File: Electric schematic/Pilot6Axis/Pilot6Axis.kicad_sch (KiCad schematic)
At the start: 63 parts, among them IC1 ESP32-WROOM-32U, IC2 LM27313XMFX_NOPB, J1 BTN1, J10 Power switch, J11 TP4056, J12 OLED, J13 USB_C_Receptacle_USB2.0_16P, J14 BTN9, J15 BTN11, J16 BTN10, J2 BTN2, J3 BTN3, J4 BTN4, J5 BTN5, J6 BTN6, J7 BTN7, J8 BTN8, J9 BAT, Q1 Q_NPN_EBC, Q2 Q_NPN_EBC, SW1 SW_Push, SW2 SW_Push, U1 JOYSTICK1, U2 JOYSTICK2, U3 AMS1117-3.3, U4 USBLC6-2SC6, U5 CP2102N-Axx-xQFN28

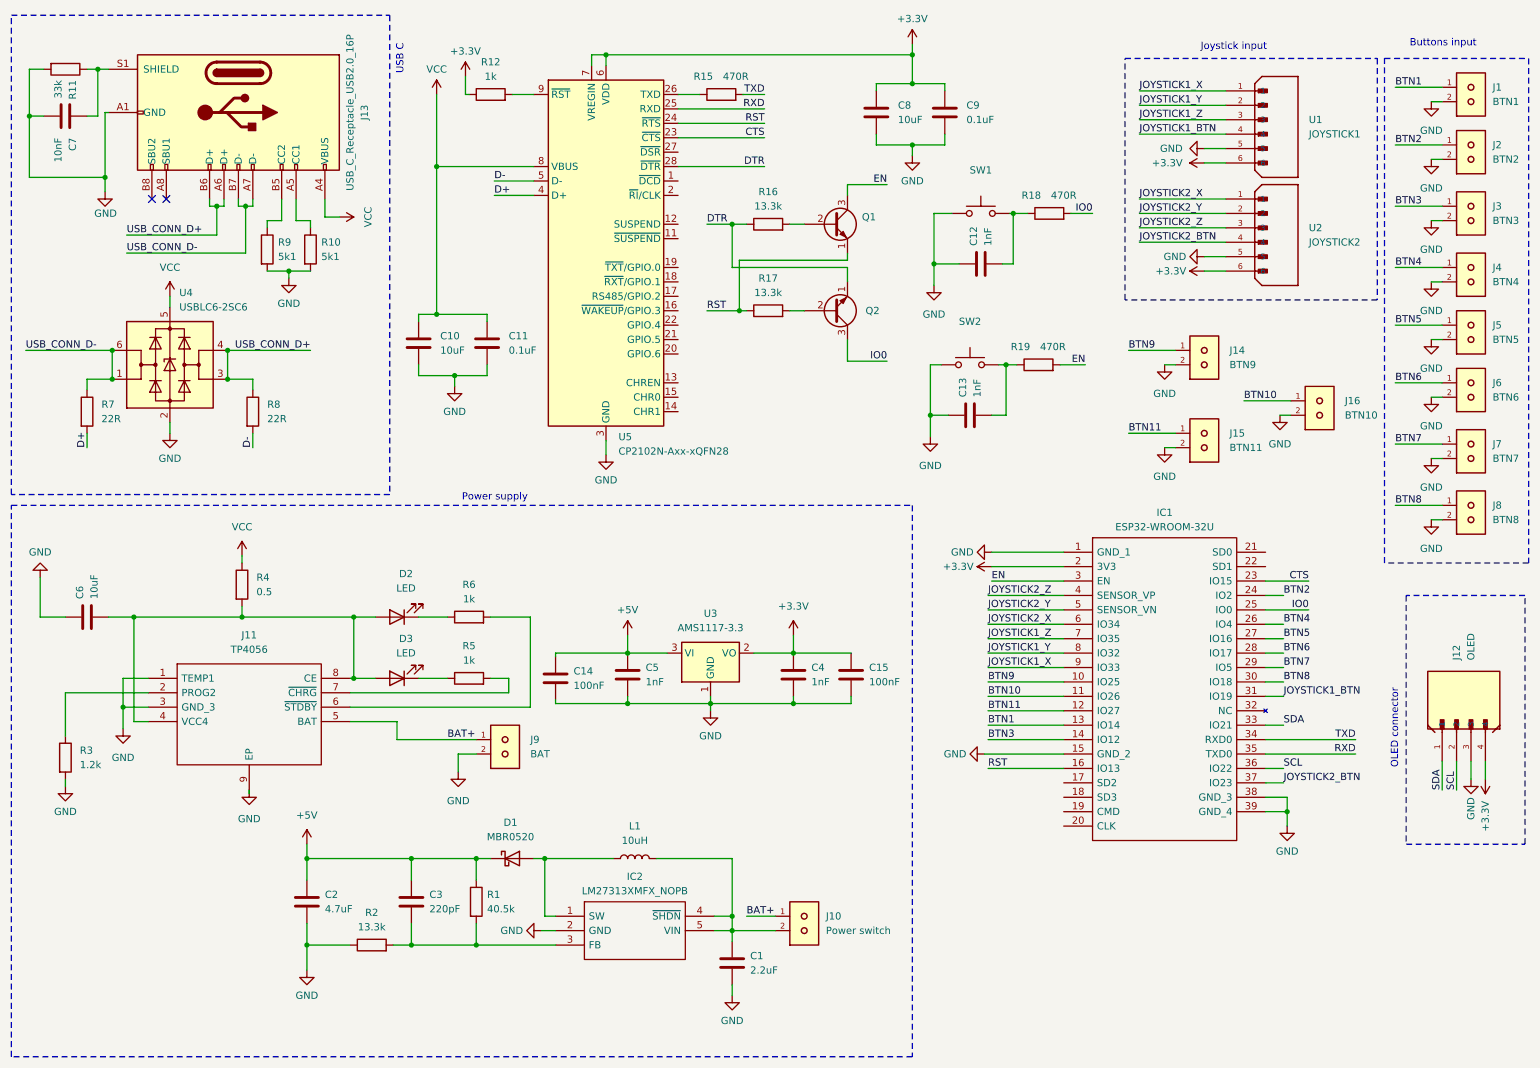
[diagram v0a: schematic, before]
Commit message: Update pilot PCB versin 1.0
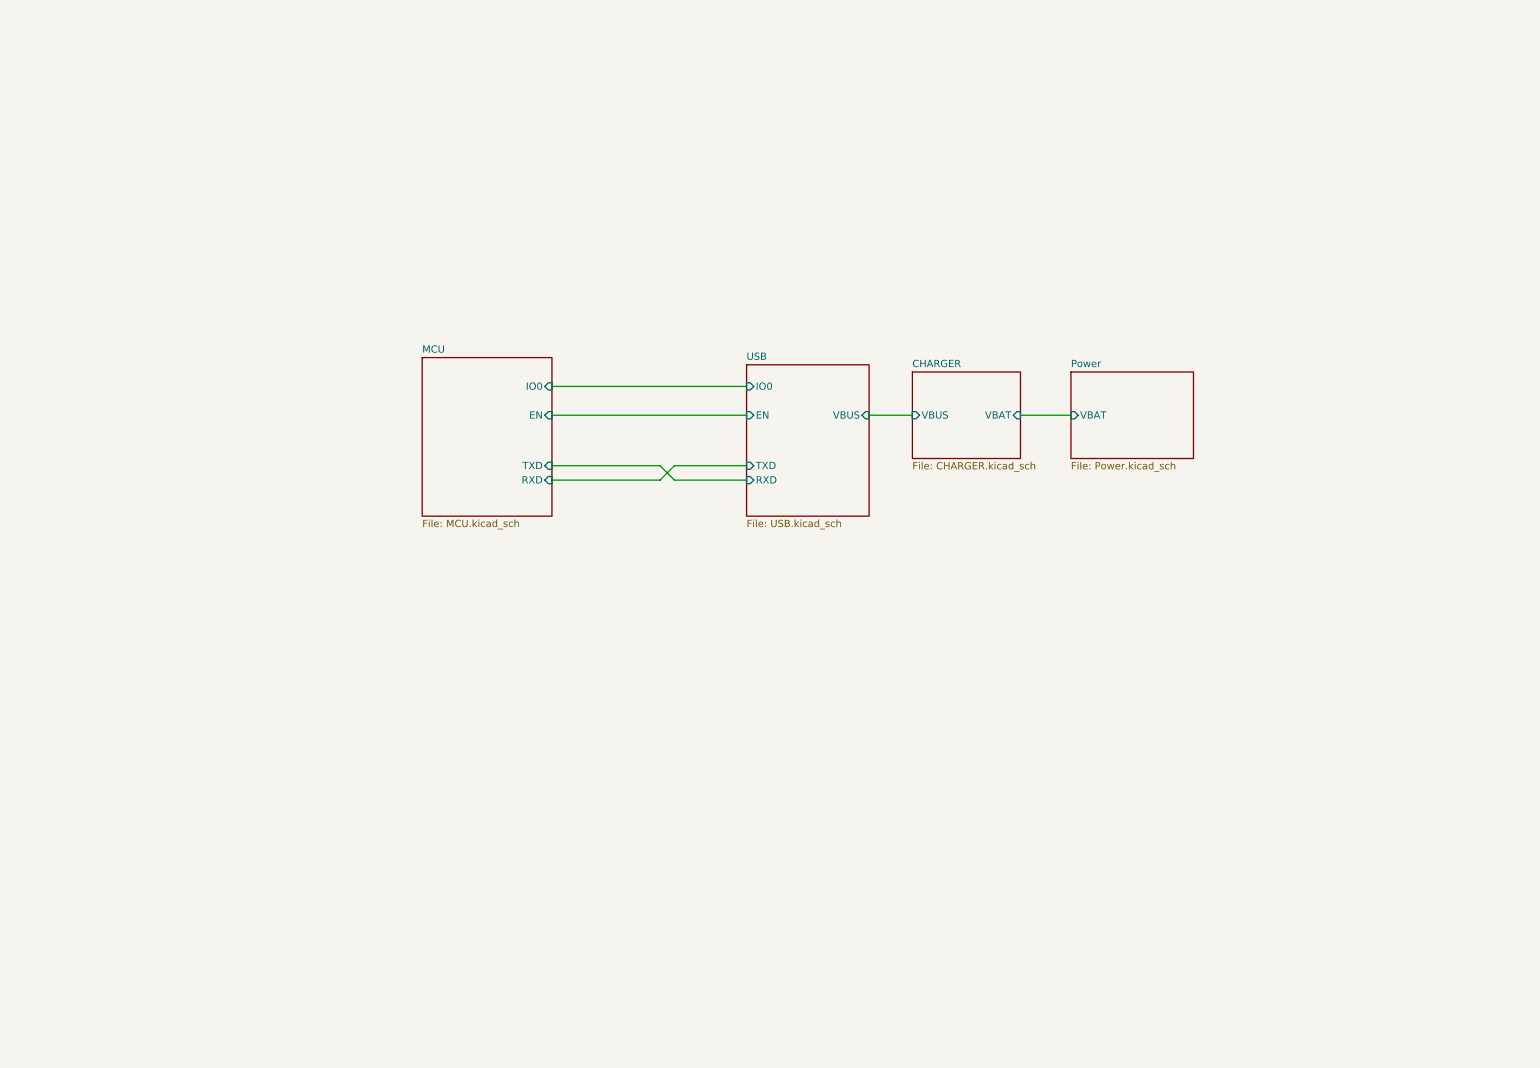
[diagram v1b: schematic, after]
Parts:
- removed C1: 2.2uF, Capacitor_SMD:C_0603_1608Metric, symbol Device:C
- removed C10, C8: 10uF, Resistor_SMD:R_0603_1608Metric, symbol Device:C
- removed C11, C9: 0.1uF, Resistor_SMD:R_0603_1608Metric, symbol Device:C
- removed C12, C13, C4, C5: 1nF, Capacitor_SMD:C_0603_1608Metric, symbol Device:C
- removed C14, C15: 100nF, Capacitor_SMD:C_0603_1608Metric, symbol Device:C
- removed C2: 4.7uF, Capacitor_SMD:C_0603_1608Metric, symbol Device:C
- removed C3: 220pF, Capacitor_SMD:C_0603_1608Metric, symbol Device:C
- removed C6: 10uF, Capacitor_SMD:C_0603_1608Metric, symbol Device:C
- removed C7: 10nF, Resistor_SMD:R_0603_1608Metric, symbol Device:C
- removed D1: MBR0520, Diode_SMD:D_0603_1608Metric, symbol Device:D_Schottky
- removed D2, D3: LED, LED_SMD:LED_0603_1608Metric, symbol Device:LED
- removed IC1: ESP32-WROOM-32U, ESP32-WROOM-32U:ESP32WROOM32D, symbol ESP32-WROOM-32U:ESP32-WROOM-32U
- removed IC2: LM27313XMFX_NOPB, KLM27313XMF_NOPB:SOT95P280X145-5N, symbol LM27313XMFX_NOPB:LM27313XMFX_NOPB
- removed J1: BTN1, molex-2pin:HDRV2W64P254_1X2_580X508X1170P, symbol molex-2pin:22-27-2021
- removed J10: Power switch, molex-2pin:HDRV2W64P254_1X2_580X508X1170P, symbol molex-2pin:22-27-2021
- removed J11: TP4056, TP4056:SOIC127P600X175-9N, symbol TP4056:TP4056
- removed J12: OLED, Connector_PinSocket_2.54mm:PinSocket_2x02_P2.54mm_Vertical, symbol molex-4pin:22232041
- removed J13: USB_C_Receptacle_USB2.0_16P, Connector_USB:USB_C_Receptacle_HCTL_HC-TYPE-C-16P-01A, symbol Connector:USB_C_Receptacle_USB2.0_16P
- removed J14: BTN9, molex-2pin:HDRV2W64P254_1X2_580X508X1170P, symbol molex-2pin:22-27-2021
- removed J15: BTN11, molex-2pin:HDRV2W64P254_1X2_580X508X1170P, symbol molex-2pin:22-27-2021
- removed J16: BTN10, molex-2pin:HDRV2W64P254_1X2_580X508X1170P, symbol molex-2pin:22-27-2021
- removed J2: BTN2, molex-2pin:HDRV2W64P254_1X2_580X508X1170P, symbol molex-2pin:22-27-2021
- removed J3: BTN3, molex-2pin:HDRV2W64P254_1X2_580X508X1170P, symbol molex-2pin:22-27-2021
- removed J4: BTN4, molex-2pin:HDRV2W64P254_1X2_580X508X1170P, symbol molex-2pin:22-27-2021
- removed J5: BTN5, molex-2pin:HDRV2W64P254_1X2_580X508X1170P, symbol molex-2pin:22-27-2021
- removed J6: BTN6, molex-2pin:HDRV2W64P254_1X2_580X508X1170P, symbol molex-2pin:22-27-2021
- removed J7: BTN7, molex-2pin:HDRV2W64P254_1X2_580X508X1170P, symbol molex-2pin:22-27-2021
- removed J8: BTN8, molex-2pin:HDRV2W64P254_1X2_580X508X1170P, symbol molex-2pin:22-27-2021
- removed J9: BAT, molex-2pin:HDRV2W64P254_1X2_580X508X1170P, symbol molex-2pin:22-27-2021
- removed L1: 10uH, Inductor_SMD:L_APV_ANR4010, symbol Device:L
- removed Q1, Q2: Q_NPN_EBC, S8050:SOT95P240X115-3N, symbol Device:Q_NPN_EBC
- removed R1: 40.5k, Resistor_SMD:R_0603_1608Metric, symbol Device:R
- removed R10, R9: 5k1, Resistor_SMD:R_0603_1608Metric, symbol Device:R
- removed R11: 33k, Resistor_SMD:R_0603_1608Metric, symbol Device:R
- removed R12, R5, R6: 1k, Resistor_SMD:R_0603_1608Metric, symbol Device:R
- removed R15, R18, R19: 470R, Resistor_SMD:R_0603_1608Metric, symbol Device:R
- removed R16, R17, R2: 13.3k, Resistor_SMD:R_0603_1608Metric, symbol Device:R
- removed R3: 1.2k, Resistor_SMD:R_0603_1608Metric, symbol Device:R
- removed R4: 0.5, Resistor_SMD:R_0603_1608Metric, symbol Device:R
- removed R7, R8: 22R, Resistor_SMD:R_0603_1608Metric, symbol Device:R
- removed SW1, SW2: SW_Push, TS-1088R-02026:TS1088R02026, symbol Switch:SW_Push
- removed U1: JOYSTICK1, Connector_PinSocket_2.54mm:PinSocket_2x03_P2.54mm_Vertical, symbol molex-6pin:22-27-2061
- removed U2: JOYSTICK2, Connector_PinSocket_2.54mm:PinSocket_2x03_P2.54mm_Vertical, symbol molex-6pin:22-27-2061
- removed U3: AMS1117-3.3, Package_TO_SOT_SMD:SOT-223-3_TabPin2, symbol Regulator_Linear:AMS1117-3.3
- removed U4: USBLC6-2SC6, Package_TO_SOT_SMD:SOT-23-6, symbol Power_Protection:USBLC6-2SC6
- removed U5: CP2102N-Axx-xQFN28, Package_DFN_QFN:QFN-28-1EP_5x5mm_P0.5mm_EP3.35x3.35mm, symbol Interface_USB:CP2102N-Axx-xQFN28
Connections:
- no-connect marks 2 -> 0
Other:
- added sheet CHARGER (CHARGER.kicad_sch)
- added sheet MCU (MCU.kicad_sch)
- added sheet Power (Power.kicad_sch)
- added sheet USB (USB.kicad_sch)
- note removed: "Buttons input"
- note removed: "Joystick input"
- note removed: "OLED connector"
- note removed: "Power supply"
- note removed: "USB C"
